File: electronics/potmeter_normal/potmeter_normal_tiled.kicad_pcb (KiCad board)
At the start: 2 copper layers, 97 x 97 mm, 175 parts, among them J1 W, J2 R2, J3 R1, J4 R2

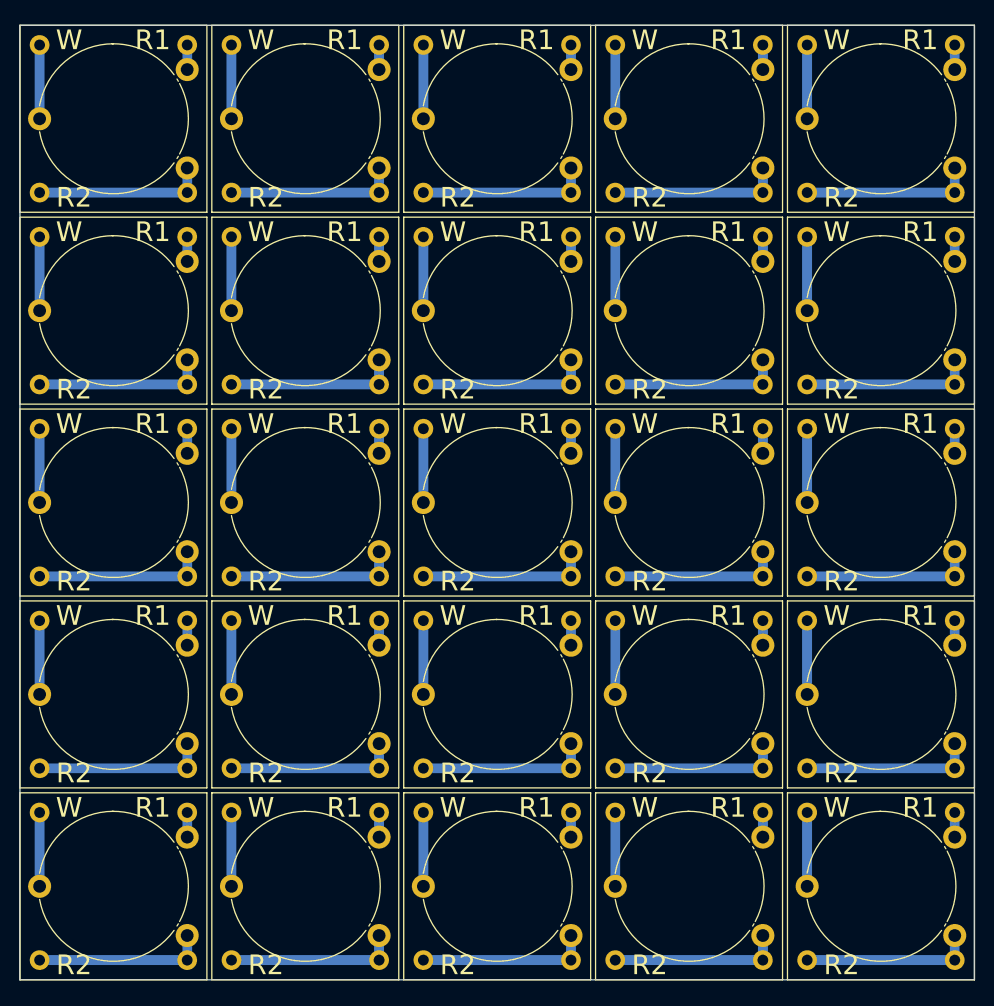
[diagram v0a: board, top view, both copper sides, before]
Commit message: reduced tiled sizes and some minor changes
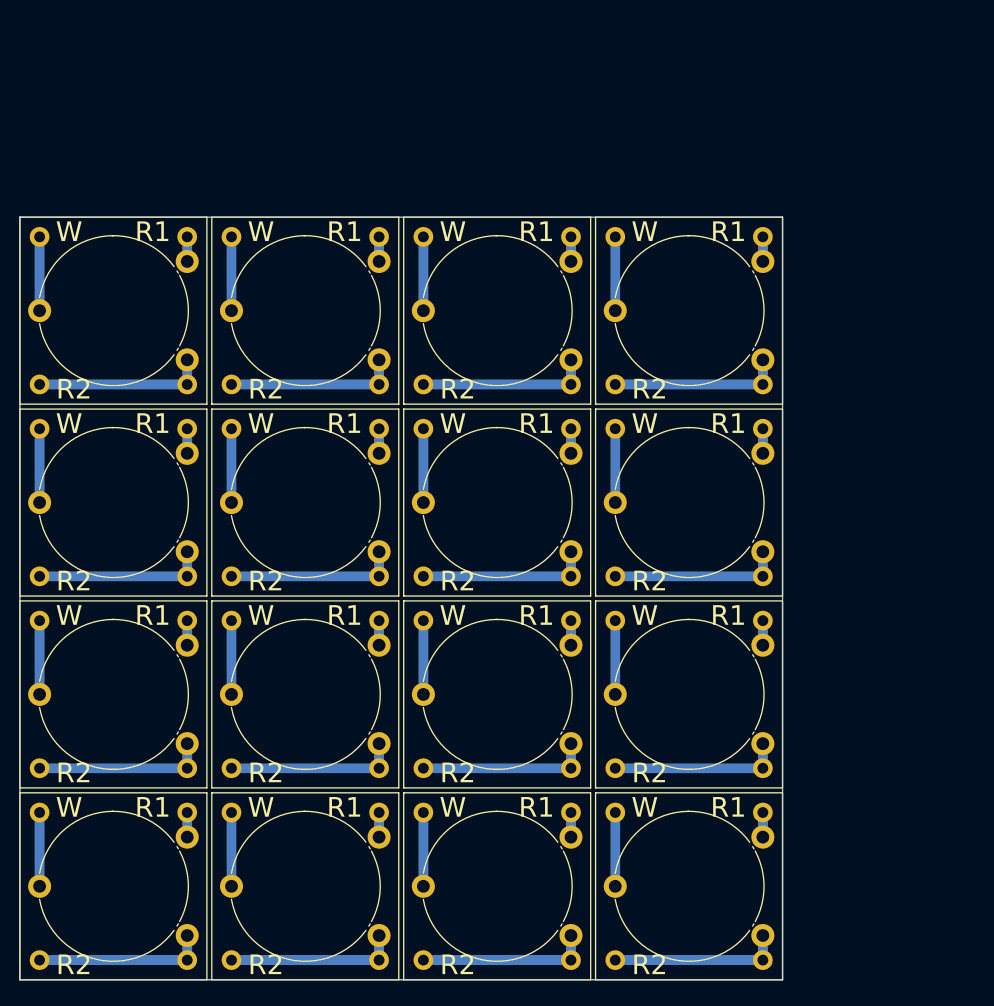
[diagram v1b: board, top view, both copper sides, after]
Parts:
- removed the J1 at (91.0, 55.0)
- removed the J1 at (130.0, 55.0)
- removed the J1 at (110.5, 55.0)
- removed the J1 at (130.0, 133.0)
- removed the J1 at (130.0, 94.0)
- removed the J1 at (52.0, 55.0)
- removed the J1 at (71.5, 55.0)
- removed the J1 at (130.0, 74.5)
- removed the J1 at (130.0, 113.5)
- removed the J2 at (130.0, 89.5)
- removed the J2 at (110.5, 70.0)
- removed the J2 at (130.0, 148.0)
- removed the J2 at (71.5, 70.0)
- removed the J2 at (91.0, 70.0)
- removed the J2 at (130.0, 128.5)
- removed the J2 at (130.0, 109.0)
- removed the J2 at (52.0, 70.0)
- removed the J2 at (130.0, 70.0)
- removed the J3 at (67.0, 55.0)
- removed the J3 at (145.0, 74.5)
- removed the J3 at (145.0, 133.0)
- removed the J3 at (145.0, 113.5)
- removed the J3 at (86.5, 55.0)
- removed the J3 at (125.5, 55.0)
- removed the J3 at (145.0, 55.0)
- removed the J3 at (145.0, 94.0)
- removed the J3 at (106.0, 55.0)
- removed the J4 at (145.0, 148.0)
- removed the J4 at (145.0, 109.0)
- removed the J4 at (106.0, 70.0)
- removed the J4 at (67.0, 70.0)
- removed the J4 at (86.5, 70.0)
- removed the J4 at (145.0, 128.5)
- removed the J4 at (145.0, 89.5)
- removed the J4 at (145.0, 70.0)
- removed the J4 at (125.5, 70.0)
- removed the N1 at (98.5, 65.0)
- removed the N1 at (137.5, 65.0)
- removed the N1 at (137.5, 104.0)
- removed the N1 at (59.5, 65.0)
- removed the N1 at (137.5, 143.0)
- removed the N1 at (79.0, 65.0)
- removed the N1 at (118.0, 65.0)
- removed the N1 at (137.5, 84.5)
- removed the N1 at (137.5, 123.5)
- removed the N2 at (79.0, 61.5)
- removed the N2 at (118.0, 61.5)
- removed the N2 at (98.5, 61.5)
- removed the N2 at (137.5, 120.0)
- removed the N2 at (137.5, 61.5)
- removed the N2 at (137.5, 81.0)
- removed the N2 at (137.5, 100.5)
- removed the N2 at (137.5, 139.5)
- removed the N2 at (59.5, 61.5)
- removed the RV1 at (67.0, 57.5)
- removed the RV1 at (145.0, 116.0)
- removed the RV1 at (145.0, 57.5)
- removed the RV1 at (106.0, 57.5)
- removed the RV1 at (145.0, 135.5)
- removed the RV1 at (145.0, 96.5)
- removed the RV1 at (86.5, 57.5)
- removed the RV1 at (125.5, 57.5)
- removed the RV1 at (145.0, 77.0)
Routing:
- net Net-(J2-Pin_1): track 437.5 -> 280.0 mm
- net Net-(J1-Pin_1): track 187.5 -> 120.0 mm
- net Net-(J3-Pin_1): track 62.5 -> 40.0 mm
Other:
- board size 97 x 97 mm -> 77.5 x 77.5 mm
